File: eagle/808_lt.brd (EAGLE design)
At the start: 100 x 80 mm, 52 parts, among them IC1 TL071P, IC2 TL072P, Q1 2N3904, Q2 2N3906, Q3 2N3904, SW8 MSS42_SW_4PDT

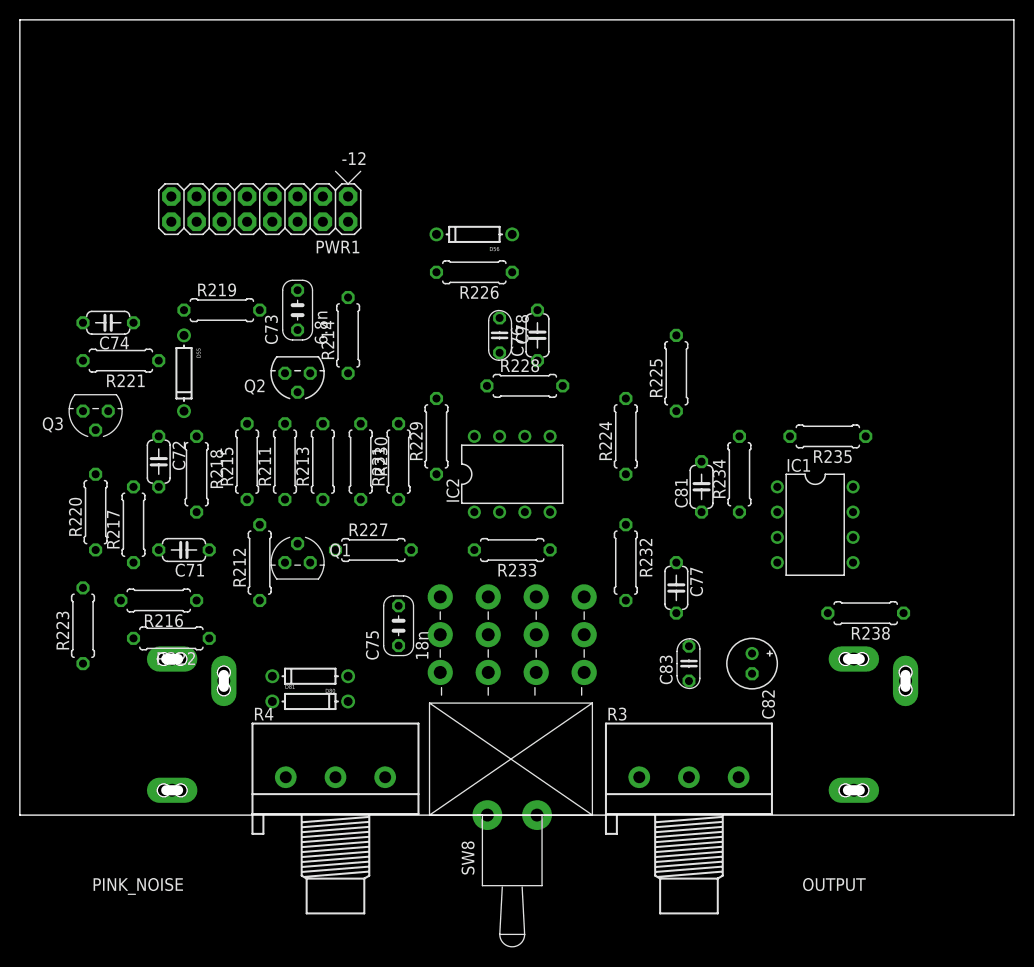
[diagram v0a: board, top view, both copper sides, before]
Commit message: routing in low 90s
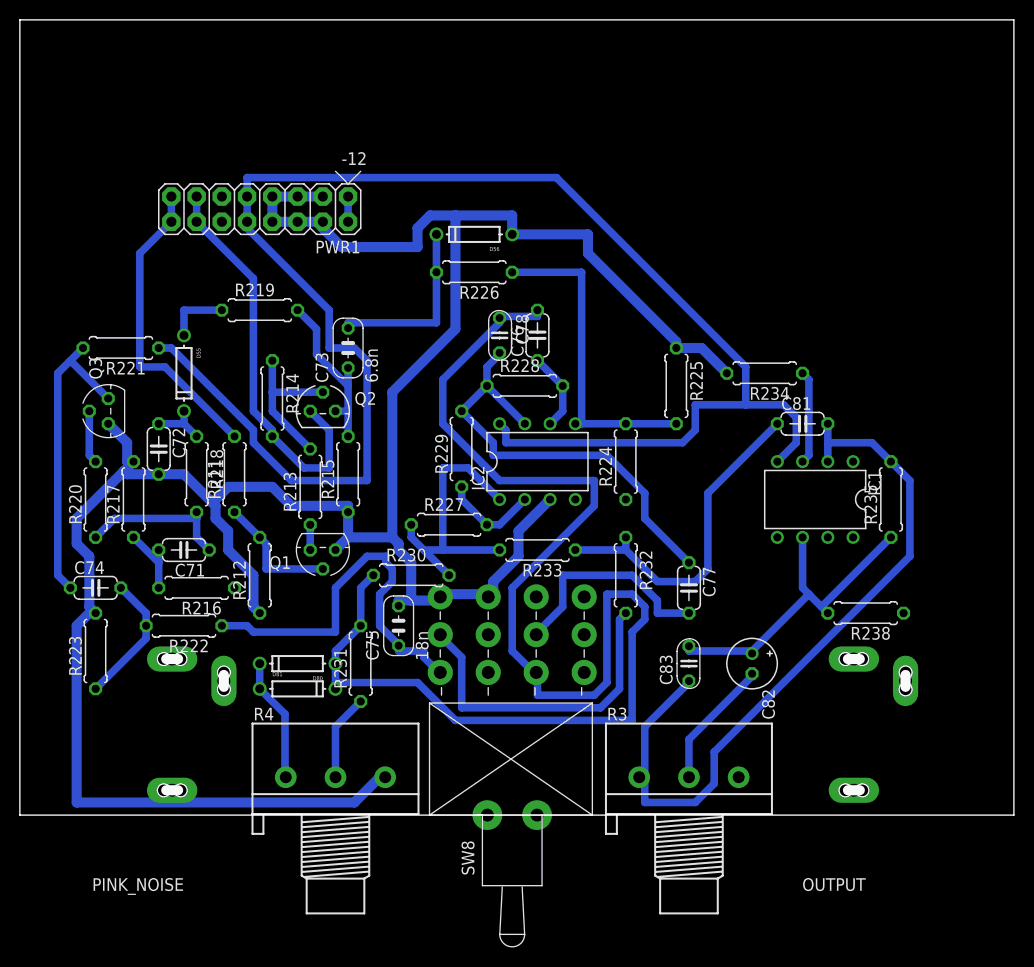
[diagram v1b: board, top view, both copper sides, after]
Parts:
- moved C74 26.7 mm to (7.62, 22.9), turned to 0 degrees
- moved R231 20.7 mm to (34.3, 15.2)
- moved R230 12.5 mm to (39.4, 24.1), turned to 0 degrees
- moved C81 12.0 mm to (78.7, 39.4), turned to 0 degrees
- moved R234 10.5 mm to (74.9, 44.5), turned to 180 degrees
- moved R215 10.2 mm to (33.0, 34.3)
- moved R214 9.92 mm to (25.4, 41.9), turned to 270 degrees
- moved R235 8.98 mm to (87.6, 31.8), turned to 90 degrees
- moved R227 8.03 mm to (43.2, 29.2)
- moved C73 6.35 mm to (33.0, 47.0)
- moved R211 5.24 mm to (21.6, 34.3)
- moved Q2 4.58 mm to (30.5, 40.6), turned to 0 degrees
- moved R216 4.02 mm to (17.8, 22.9)
- moved R219 3.81 mm to (24.1, 50.8)
- moved R229 2.84 mm to (44.5, 36.8)
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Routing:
- net GND: track 0.00 -> 254.7 mm
- net +15V: track 0.00 -> 166.3 mm
- net N$251: track 0.00 -> 138.5 mm
- net N$260: track 0.00 -> 74.7 mm
- net N$253: track 0.00 -> 44.2 mm
- net TRIG: track 0.00 -> 40.8 mm
- net N$264: track 0.00 -> 39.1 mm
- net N$259: track 0.00 -> 33.9 mm
- net N$262: track 0.00 -> 33.7 mm
- net N$273: track 0.00 -> 32.8 mm
- net N$39: track 0.00 -> 32.4 mm
- net N$263: track 0.00 -> 31.1 mm
- net LT: track 0.00 -> 30.9 mm
- net N$257: track 0.00 -> 29.6 mm
- net N$271: track 0.00 -> 22.1 mm
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
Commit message: closer
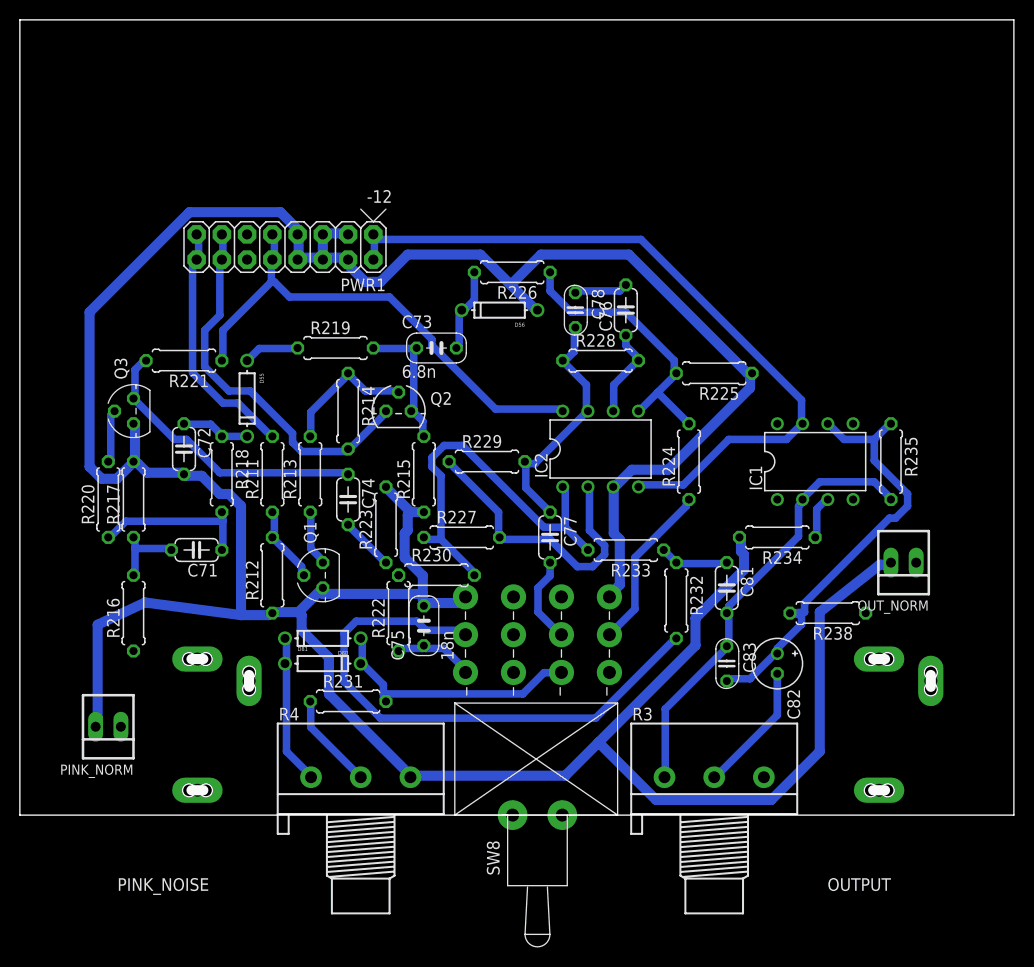
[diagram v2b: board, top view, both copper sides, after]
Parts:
- added OUT_NORM, PINK_NORM: 22-23-2021, con-molex:22-23-2021
- moved R223 31.9 mm to (36.8, 29.2)
- moved C74 26.9 mm to (33.0, 31.8), turned to 270 degrees
- moved R222 21.6 mm to (38.1, 20.3), turned to 90 degrees
- moved C81 18.2 mm to (71.1, 22.9), turned to 270 degrees
- moved R234 16.6 mm to (76.2, 27.9)
- moved C77 14.9 mm to (53.3, 27.9)
- moved C76 9.25 mm to (61.0, 50.8)
- moved R233 8.89 mm to (61.0, 26.7)
- moved C73 8.89 mm to (41.9, 47.0), turned to 0 degrees
- moved R219 8.52 mm to (31.8, 47.0)
- moved C78 8.03 mm to (55.9, 50.8)
- moved D56 8.03 mm to (48.3, 50.8)
- moved R228 8.03 mm to (58.4, 45.7)
- moved R214 7.73 mm to (33.0, 40.6)
- moved Q2 7.62 mm to (38.1, 40.6)
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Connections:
- new net N$3: OUTPUT.P$2, OUT_NORM.1
- new net N$4: PINK_NOISE.P$2, PINK_NORM.1
- net GND: now also OUT_NORM.2, PINK_NORM.2, SW8.P$12; no longer SW8.P$6
- net N$111: now also SW8.P$11; no longer SW8.P$5
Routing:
- net +15V: track 166.3 -> 50.2 mm
- net N$251: track 138.5 -> 31.8 mm
- net GND: track 254.7 -> 357.0 mm
- net -15V: track 2.54 -> 74.1 mm
- net N$264: track 39.1 -> 8.47 mm
- net N$260: track 74.7 -> 44.3 mm
- net N$259: track 33.9 -> 6.96 mm
- net N$273: track 32.8 -> 56.5 mm
- net N$256: track 9.72 -> 29.5 mm
- net N$253: track 44.2 -> 24.8 mm
- net N$111: track 0.00 -> 17.0 mm
- net N$271: track 22.1 -> 8.77 mm
- net N$262: track 33.7 -> 45.1 mm
- net N$257: track 29.6 -> 40.2 mm
- net N$250: track 18.3 -> 8.52 mm
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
